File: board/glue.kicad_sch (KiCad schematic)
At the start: 20 parts, among them J1 Conn_ARM_JTAG_SWD_10, J8 SD_Card_Receptacle, U12 GLUE, U13 SN74LVC245APW, U14 LD1117V33

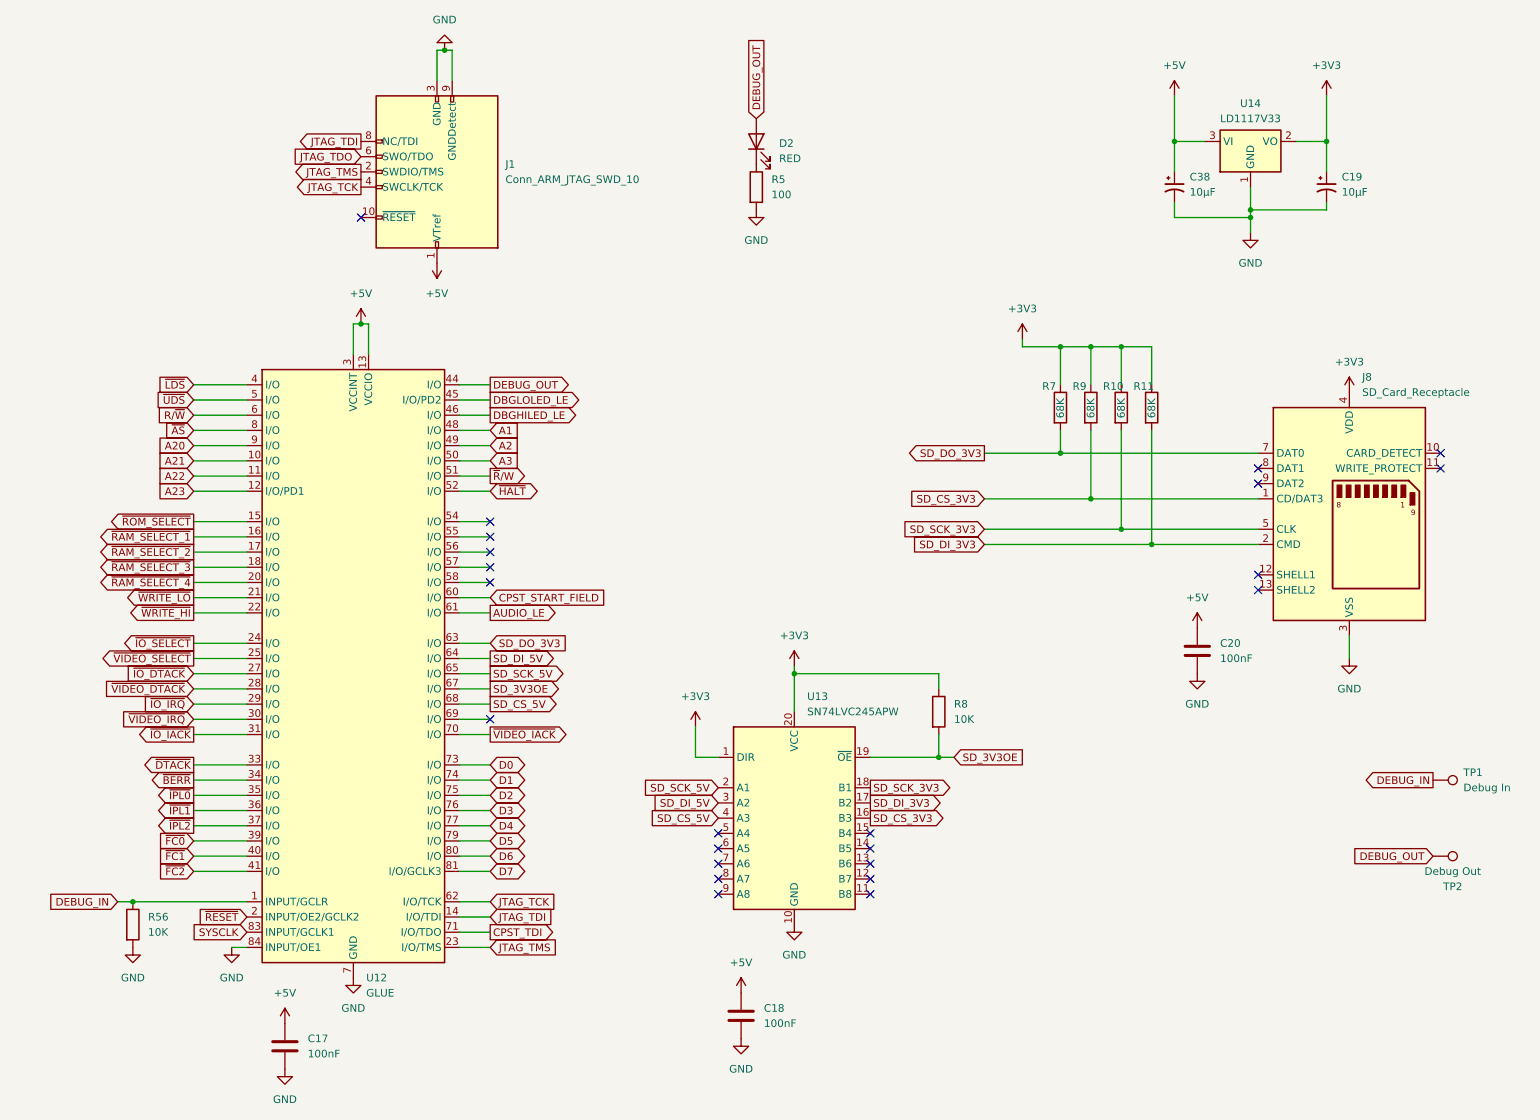
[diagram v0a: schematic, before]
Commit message: checkpoint
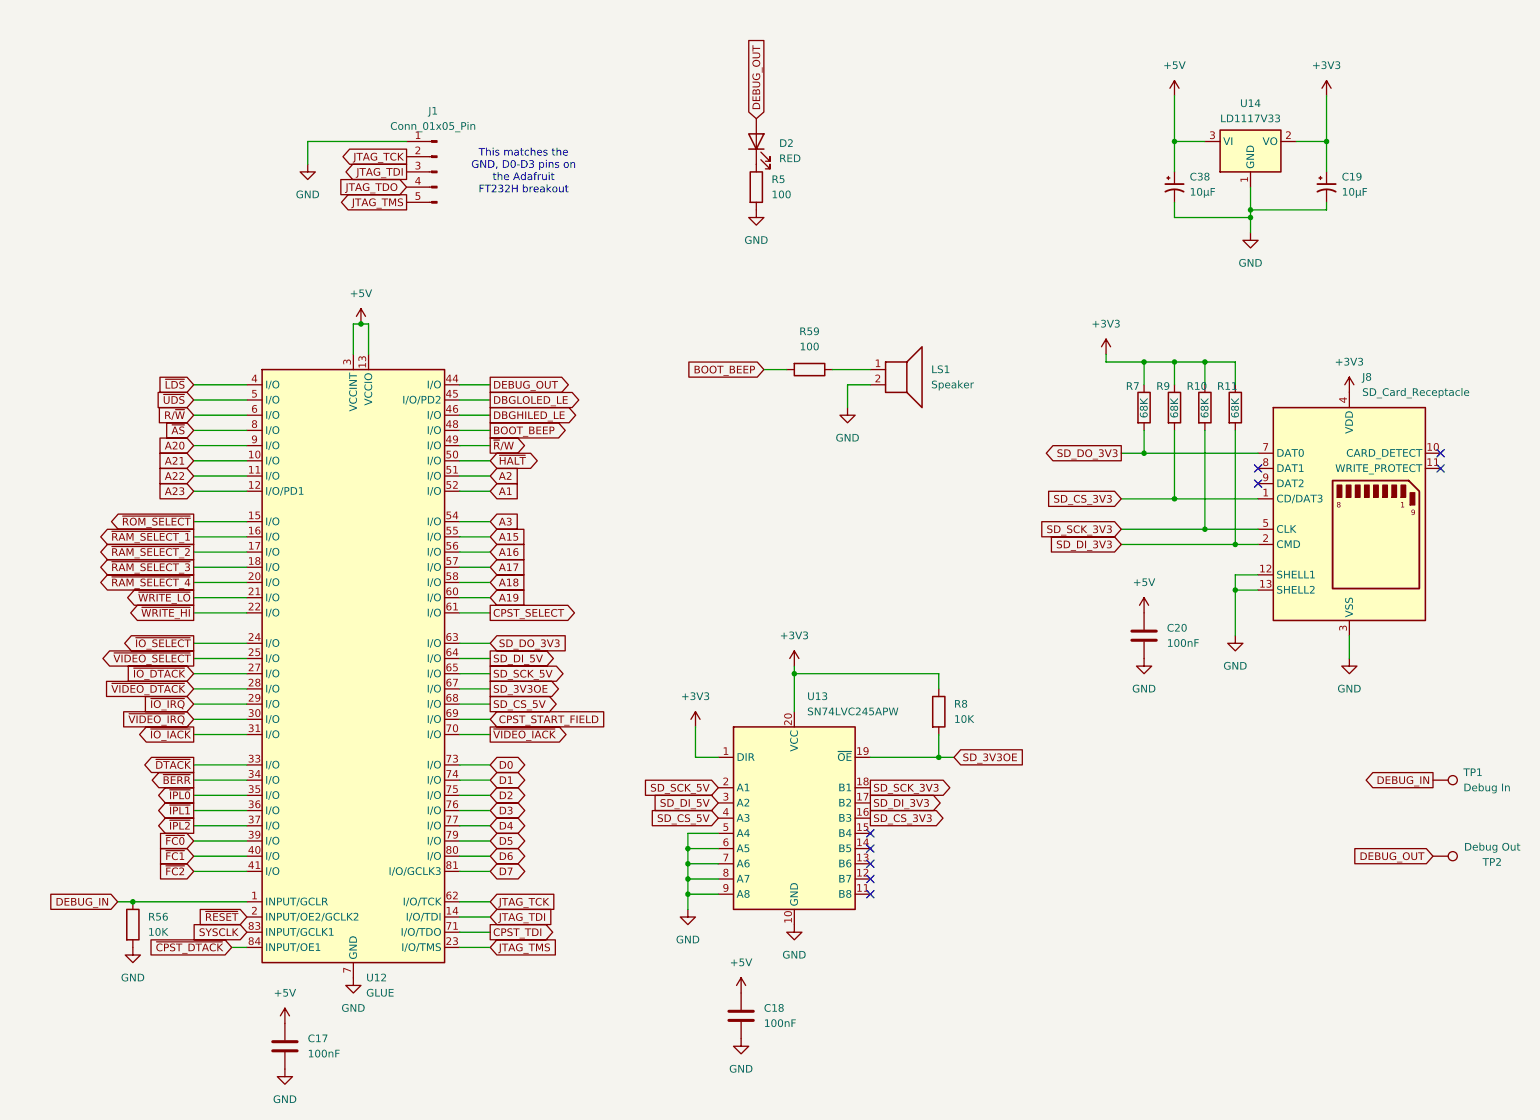
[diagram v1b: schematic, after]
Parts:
- removed J1: Conn_ARM_JTAG_SWD_10, Connector_PinHeader_1.27mm:PinHeader_2x05_P1.27mm_Vertical, symbol Connector:Conn_ARM_JTAG_SWD_10
- added J1: Conn_01x05_Pin, Connector_PinHeader_2.54mm:PinHeader_1x05_P2.54mm_Vertical, symbol Connector:Conn_01x05_Pin
- added LS1: Speaker, Buzzer_Beeper:MagneticBuzzer_StarMicronics_QMX, symbol Device:Speaker
- added R59: 100, Resistor_THT:R_Axial_DIN0207_L6.3mm_D2.5mm_P10.16mm_Horizontal, symbol Device:R
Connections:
- net A1: now also U12.52 (I/O); no longer U12.48 (I/O)
- net A2: now also U12.51 (I/O); no longer U12.49 (I/O)
- net A3: now also U12.54 (I/O); no longer U12.50 (I/O)
- net CPST_START_FIELD: now also U12.69 (I/O); no longer U12.60 (I/O)
- net GND: now also J8.12 (SHELL1), J8.13 (SHELL2), U13.5 (A4), U13.6 (A5), U13.7 (A6), U13.8 (A7), U13.9 (A8), J1.1 (Pin_1), LS1.2; no longer U12.84 (INPUT/OE1)
- net JTAG_TCK: now also J1.2 (Pin_2)
- net JTAG_TDI: now also J1.3 (Pin_3)
- net JTAG_TDO: now also J1.4 (Pin_4)
- net JTAG_TMS: now also J1.5 (Pin_5)
- net ~{HALT}: now also U12.50 (I/O); no longer U12.52 (I/O)
- net ~{R}/W: now also U12.49 (I/O); no longer U12.51 (I/O)
- net A15: now reaches U12.55 (I/O)
- net A16: now reaches U12.56 (I/O)
- net A17: now reaches U12.57 (I/O)
- net A18: now reaches U12.58 (I/O)
- net AUDIO_LE renamed CPST_SELECT
- new net: LS1.1, R59.1
- new net A19: U12.60 (I/O)
- new net BOOT_BEEP: R59.2, U12.48 (I/O)
- new net ~{CPST_DTACK}: U12.84 (INPUT/OE1)
- no-connect marks 23 -> 9
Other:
- note added: "This matches the GND, D0-D3 pins on the Adafruit FT232H breakout"
- moved on the sheet: C20, R10, R11, R7, R9

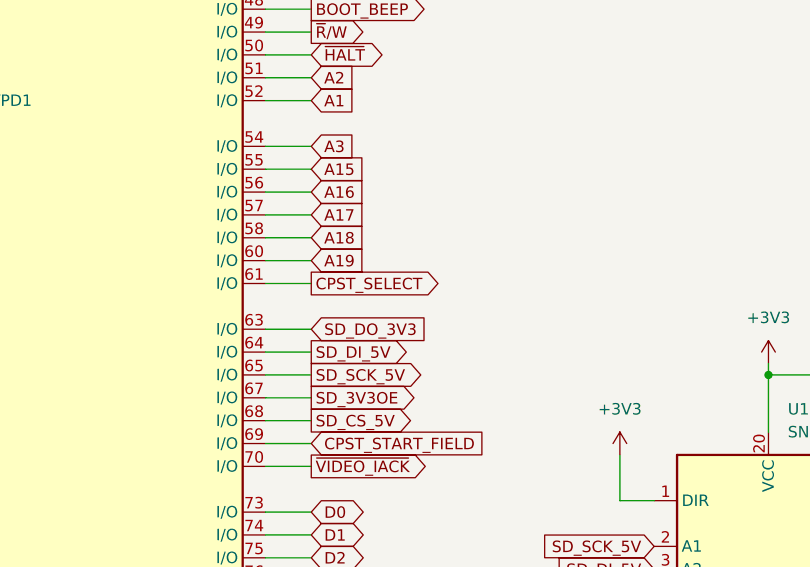
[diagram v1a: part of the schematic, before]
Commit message: checkpoint
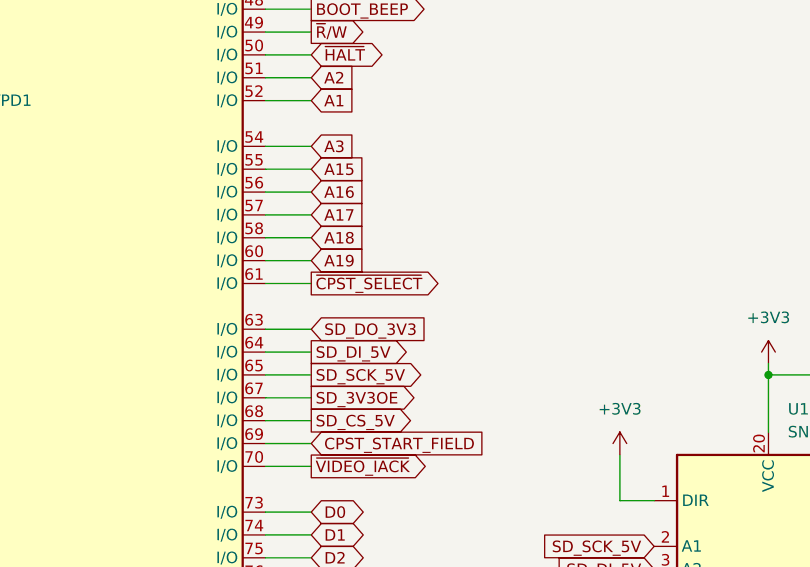
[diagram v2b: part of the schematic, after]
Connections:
- net CPST_SELECT renamed ~{CPST_SELECT}
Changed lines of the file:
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@@
+	)
+	(junction
+		(at 120.65 162.56)
+		(diameter 0)
+		(color 0 0 0 0)
 	)
 	(junction
@@
 	(junction
 		(at 120.65 154.94)
-		(diameter 0)
-		(color 0 0 0 0)
-	)
-	(junction
-		(at 120.65 162.56)
 		(diameter 0)
 		(color 0 0 0 0)
@@
 	(wire
 		(pts
+			(xy 82.55 146.05) (xy 87.63 146.05)
+		)
+		(stroke
+			(width 0)
+			(type default)
+		)
+	)
+	(wire
+		(pts
+			(xy 82.55 120.65) (xy 87.63 120.65)
+		)
+		(stroke
+			(width 0)
+			(type default)
+		)
+	)
+	(wire
+		(pts
+			(xy 82.55 102.87) (xy 87.63 102.87)
+		)
+		(stroke
+			(width 0)
+			(type default)
+		)
+	)
+	(wire
+		(pts
+			(xy 162.56 139.7) (xy 165.1 139.7)
+		)
+		(stroke
+			(width 0)
+			(type default)
+		)
+	)
+	(wire
+		(pts
+			(xy 64.77 67.31) (xy 64.77 72.39)
+		)
+		(stroke
+			(width 0)
+			(type default)
+		)
+	)
+	(wire
+		(pts
+			(xy 82.55 171.45) (xy 87.63 171.45)
+		)
+		(stroke
+			(width 0)
+			(type default)
+		)
+	)
+	(wire
+		(pts
+			(xy 38.1 151.13) (xy 46.99 151.13)
+		)
+		(stroke
+			(width 0)
+			(type default)
+		)
+	)
+	(wire
+		(pts
+			(xy 207.01 85.09) (xy 207.01 101.6)
+		)
+		(stroke
+			(width 0)
+			(type default)
+		)
+	)
+	(wire
+		(pts
+			(xy 38.1 100.33) (xy 46.99 100.33)
+		)
+		(stroke
+			(width 0)
+			(type default)
+		)
+	)
+	(wire
+		(pts
+			(xy 196.85 88.9) (xy 215.9 88.9)
+		)
+		(stroke
+			(width 0)
+			(type default)
+		)
+	)
+	(wire
+		(pts
+			(xy 120.65 154.94) (xy 120.65 157.48)
+		)
+		(stroke
+			(width 0)
+			(type default)
+		)
+	)
+	(wire
+		(pts
+			(xy 82.55 110.49) (xy 87.63 110.49)
+		)
+		(stroke
+			(width 0)
+			(type default)
+		)
+	)
+	(wire
+		(pts
+			(xy 44.45 171.45) (xy 46.99 171.45)
+		)
+		(stroke
+			(width 0)
+			(type default)
+		)
+	)
+	(wire
+		(pts
+			(xy 82.55 143.51) (xy 87.63 143.51)
+		)
+		(stroke
+			(width 0)
+			(type default)
+		)
+	)
+	(wire
+		(pts
+			(xy 25.4 163.83) (xy 27.94 163.83)
+		)
+		(stroke
+			(width 0)
+			(type default)
+		)
+	)
+	(wire
+		(pts
+			(xy 201.93 73.66) (xy 207.01 73.66)
+		)
+		(stroke
+			(width 0)
+			(type default)
+		)
+	)
+	(wire
+		(pts
 			(xy 120.65 162.56) (xy 120.65 165.1)
-		)
-		(stroke
-			(width 0)
-			(type default)
-		)
-	)
-	(wire
-		(pts
-			(xy 82.55 146.05) (xy 87.63 146.05)
-		)
-		(stroke
-			(width 0)
-			(type default)
-		)
-	)
-	(wire
-		(pts
-			(xy 82.55 120.65) (xy 87.63 120.65)
-		)
-		(stroke
-			(width 0)
-			(type default)
-		)
-	)
-	(wire
-		(pts
-			(xy 82.55 102.87) (xy 87.63 102.87)
-		)
-		(stroke
-			(width 0)
-			(type default)
-		)
-	)
-	(wire
-		(pts
-			(xy 162.56 139.7) (xy 165.1 139.7)
-		)
-		(stroke
-			(width 0)
-			(type default)
-		)
-	)
-	(wire
-		(pts
-			(xy 64.77 67.31) (xy 64.77 72.39)
-		)
-		(stroke
-			(width 0)
-			(type default)
-		)
-	)
-	(wire
-		(pts
-			(xy 82.55 171.45) (xy 87.63 171.45)
-		)
-		(stroke
-			(width 0)
-			(type default)
-		)
-	)
-	(wire
-		(pts
-			(xy 38.1 151.13) (xy 46.99 151.13)
-		)
-		(stroke
-			(width 0)
-			(type default)
-		)
-	)
-	(wire
-		(pts
-			(xy 207.01 85.09) (xy 207.01 101.6)
-		)
-		(stroke
-			(width 0)
-			(type default)
-		)
-	)
-	(wire
-		(pts
-			(xy 38.1 100.33) (xy 46.99 100.33)
-		)
-		(stroke
-			(width 0)
-			(type default)
-		)
-	)
-	(wire
-		(pts
-			(xy 196.85 88.9) (xy 215.9 88.9)
-		)
-		(stroke
-			(width 0)
-			(type default)
-		)
-	)
-	(wire
-		(pts
-			(xy 120.65 154.94) (xy 120.65 157.48)
-		)
-		(stroke
-			(width 0)
-			(type default)
-		)
-	)
-	(wire
-		(pts
-			(xy 82.55 110.49) (xy 87.63 110.49)
-		)
-		(stroke
-			(width 0)
-			(type default)
-		)
-	)
-	(wire
-		(pts
-			(xy 44.45 171.45) (xy 46.99 171.45)
-		)
-		(stroke
-			(width 0)
-			(type default)
-		)
-	)
-	(wire
-		(pts
-			(xy 82.55 143.51) (xy 87.63 143.51)
-		)
-		(stroke
-			(width 0)
-			(type default)
-		)
-	)
-	(wire
-		(pts
-			(xy 25.4 163.83) (xy 27.94 163.83)
-		)
-		(stroke
-			(width 0)
-			(type default)
-		)
-	)
-	(wire
-		(pts
-			(xy 201.93 73.66) (xy 207.01 73.66)
 		)
 		(stroke
@@
 		)
 	)
-	(global_label "CPST_SELECT"
+	(global_label "~{CPST_SELECT}"
 		(shape output)
 		(at 87.63 115.57 0)

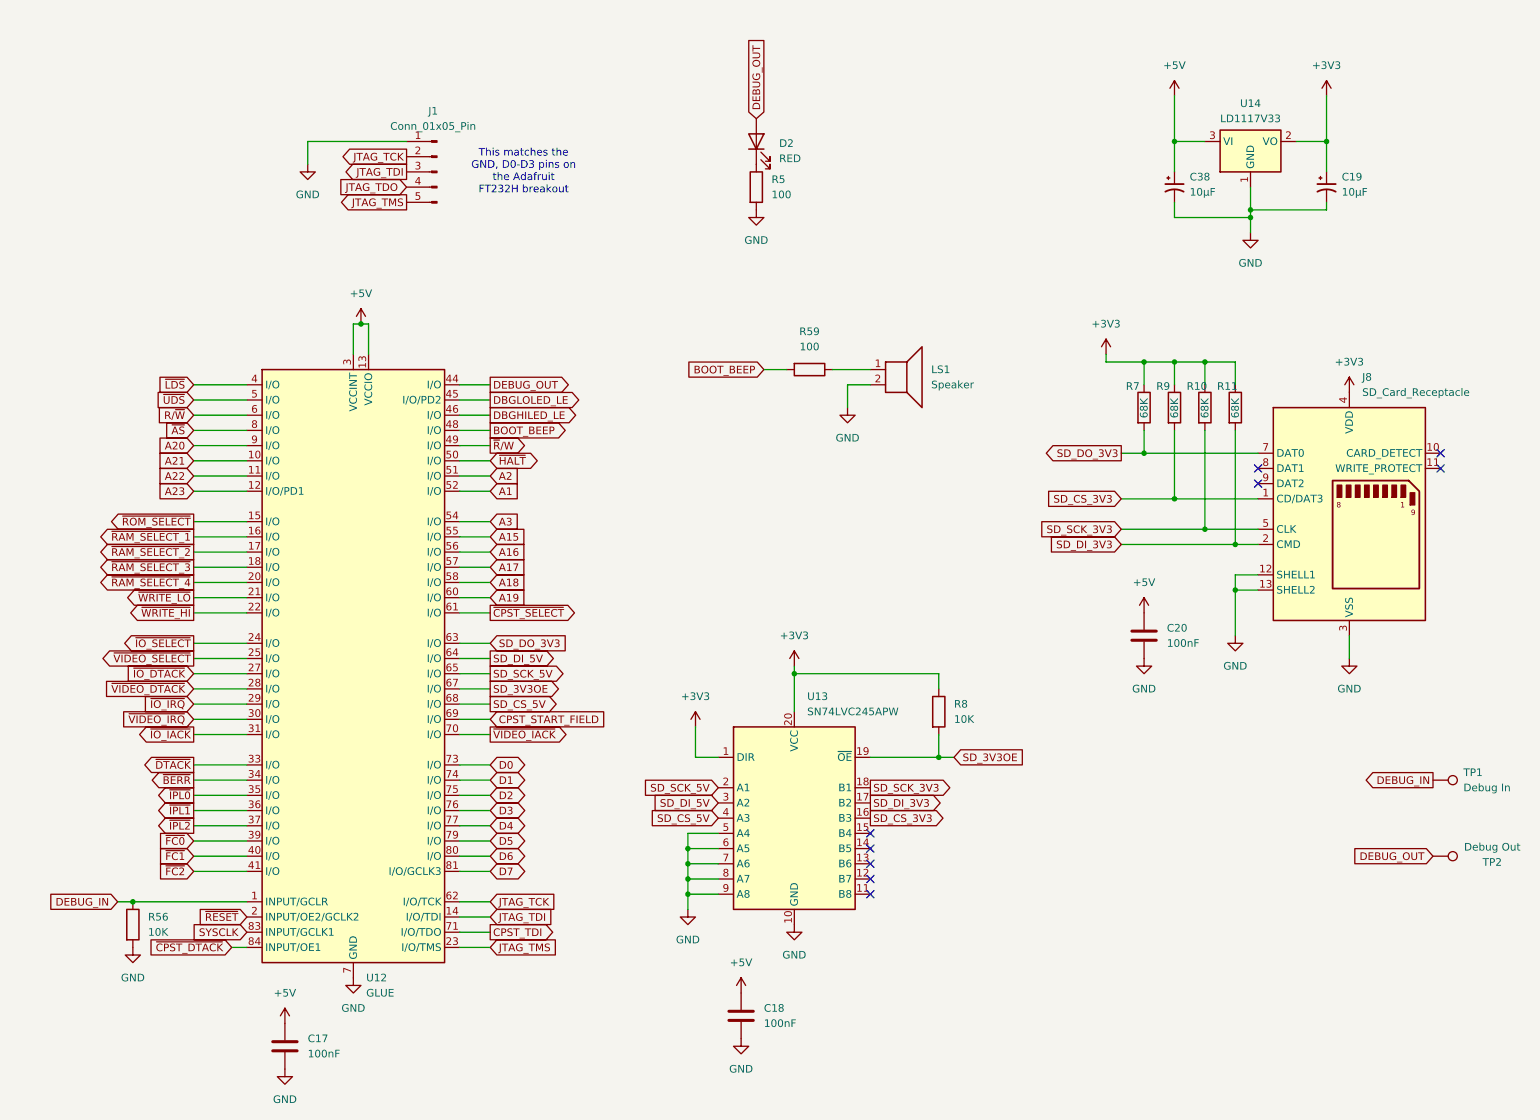
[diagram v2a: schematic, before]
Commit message: checkpoint - maybe unfinishable
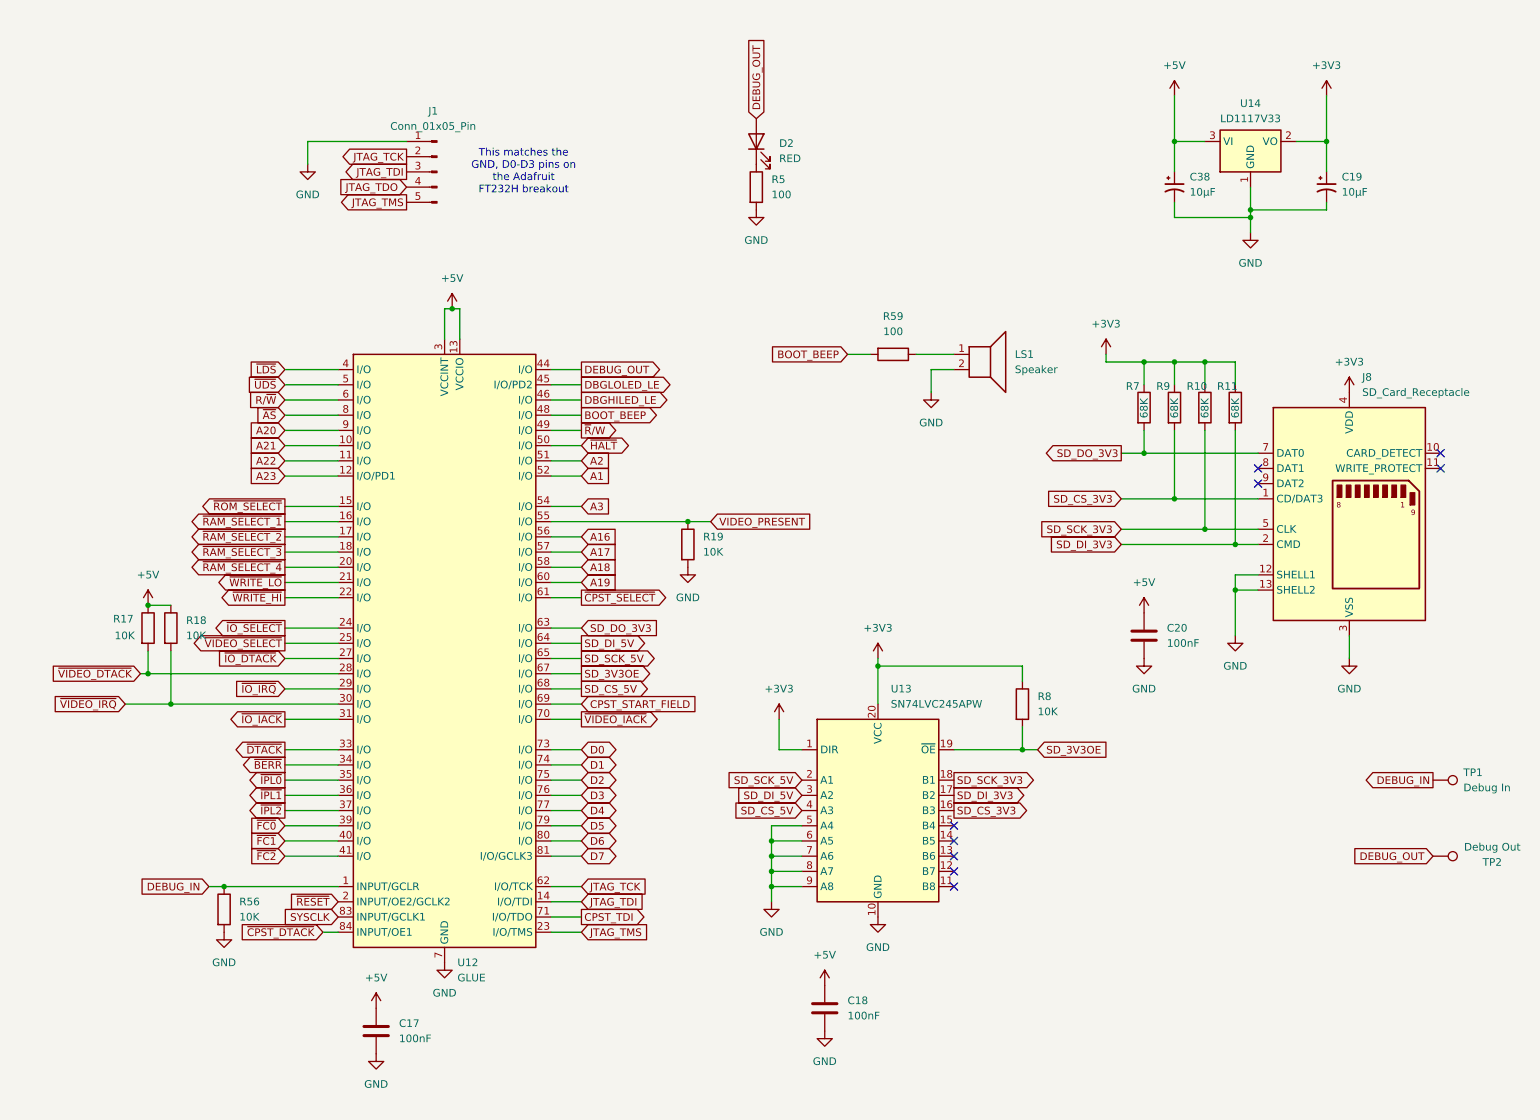
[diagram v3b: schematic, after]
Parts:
- added R17, R18, R19: 10K, Resistor_THT:R_Axial_DIN0207_L6.3mm_D2.5mm_P10.16mm_Horizontal, symbol Device:R
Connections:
- net +5V: now also R17.1, R18.1
- net GND: now also R19.2
- net ~{VIDEO_DTACK}: now also R17.2
- net ~{VIDEO_IRQ}: now also R18.2
- net A15 renamed VIDEO_PRESENT
- net VIDEO_PRESENT: now also R19.1
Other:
- moved on the sheet: C17, C18, LS1, R56, R59, R8, U12, U13
